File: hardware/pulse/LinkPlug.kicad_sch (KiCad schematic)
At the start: 4 parts, among them J1901 2x05_Horizontal, U1901 THVD24x2

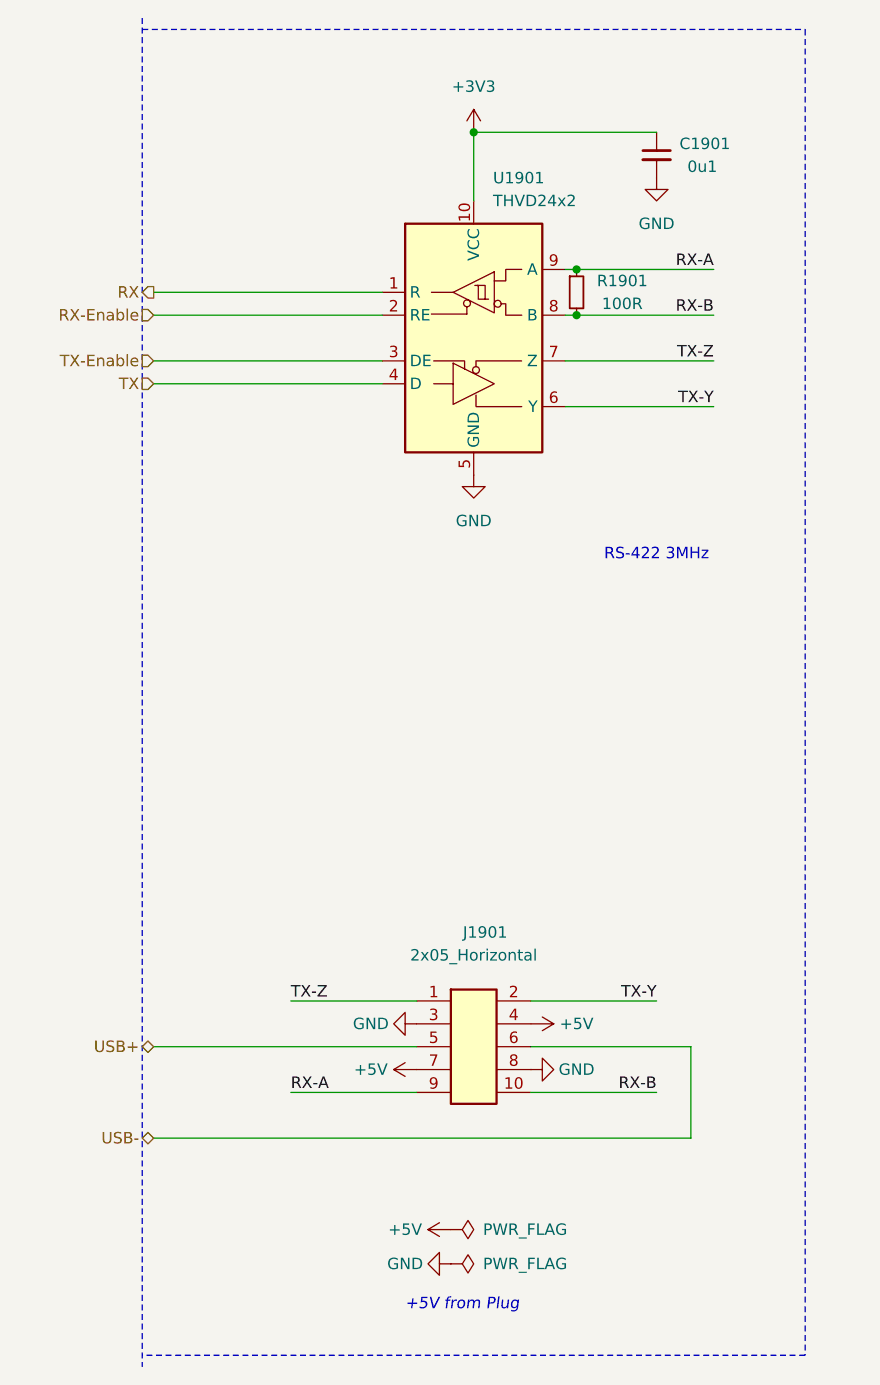
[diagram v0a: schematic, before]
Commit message: Update parts
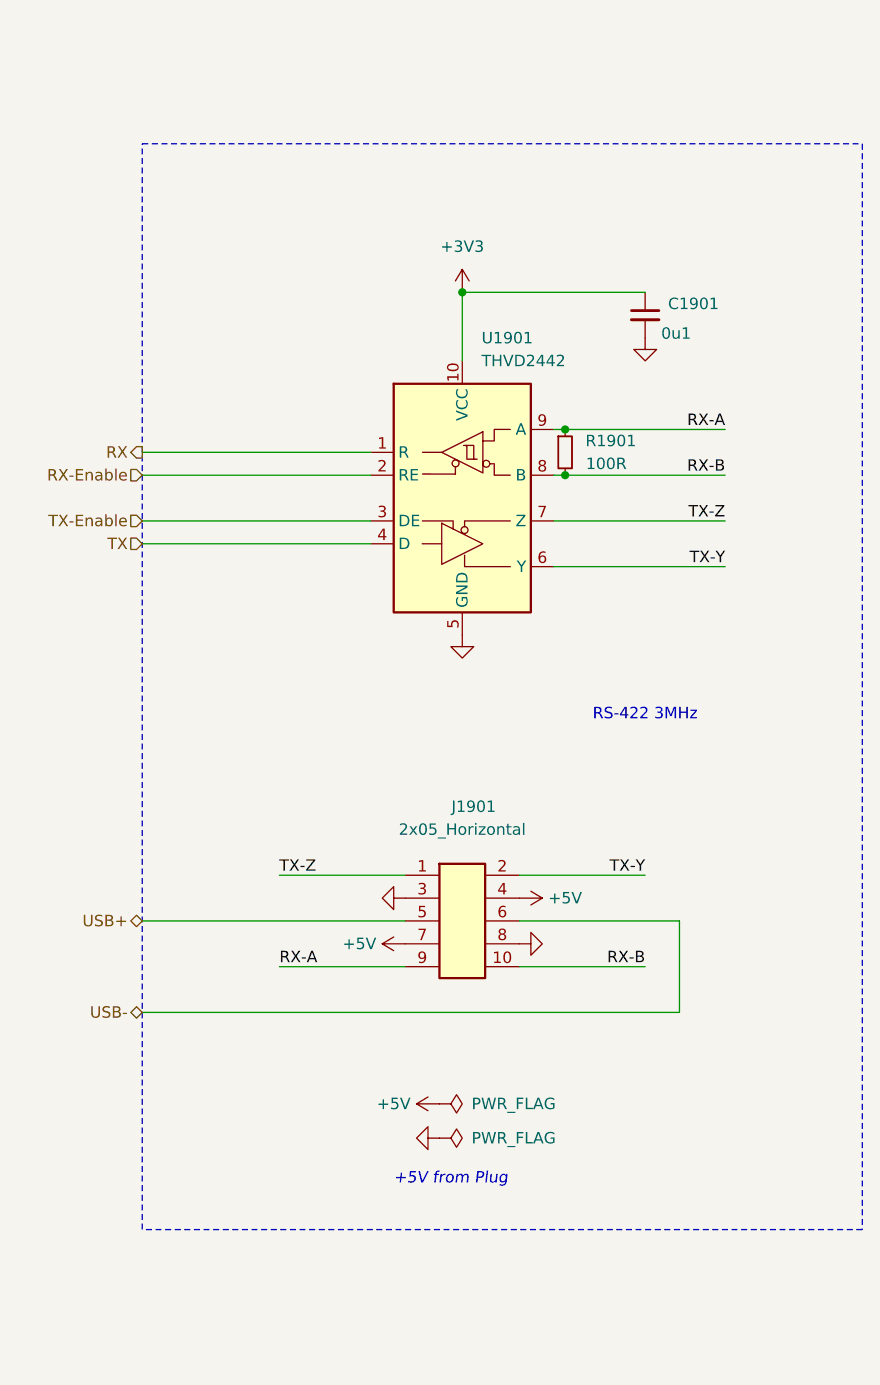
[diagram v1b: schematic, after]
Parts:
- C1901: footprint Capacitor_SMD:C_0603_1608Metric -> V2_Capacitor_SMD:C_0603; symbol Device:C_Small -> V2_Device:C_0603_0u1; Manufacturer (none) -> TDK; Mouser (none) -> 810-CGA3E2X7R1H104MA; Product (none) -> CGA3E2X7R1H104M080AA
- J1901: Manufacturer (none) -> Amphenol FCI; Mouser (none) -> 649-200211120001T4LF; Product (none) -> 20021112-00010T4LF
- R1901: footprint Resistor_SMD:R_0603_1608Metric -> V2_Resistor_SMD:R_0603; symbol Device:R_Small -> V2_Device:R_0603_100R; Manufacturer (none) -> Vishay; Mouser (none) -> 71-CRCW0603100RFKEAH; Product (none) -> CRCW0603100RFKEAHP; Rating (none) -> 330mW
- U1901: value THVD24x2 -> THVD2442; symbol V2_Interface_RS485:THVD24x2 -> V2_Interface_RS485:THVD2442; Manufacturer (none) -> Texas Instruments; Mouser (none) -> 595-THVD2442DRCR; Product (none) -> THVD2442DRCR
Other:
- moved on the sheet: C1901, J1901, R1901, U1901
